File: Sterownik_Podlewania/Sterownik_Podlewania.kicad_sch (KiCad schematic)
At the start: 26 parts, among them J10 Conn_01x06_Socket, J11 Conn_01x06_Socket, J3 Conn_01x05_Pin, J4 Conn_01x05_Pin, J5 Conn_01x03_Pin, J7 Conn_01x05_Socket, J8 Conn_01x04_Socket, J9 Conn_01x06_Socket, U1 ESP32-DEVKITC

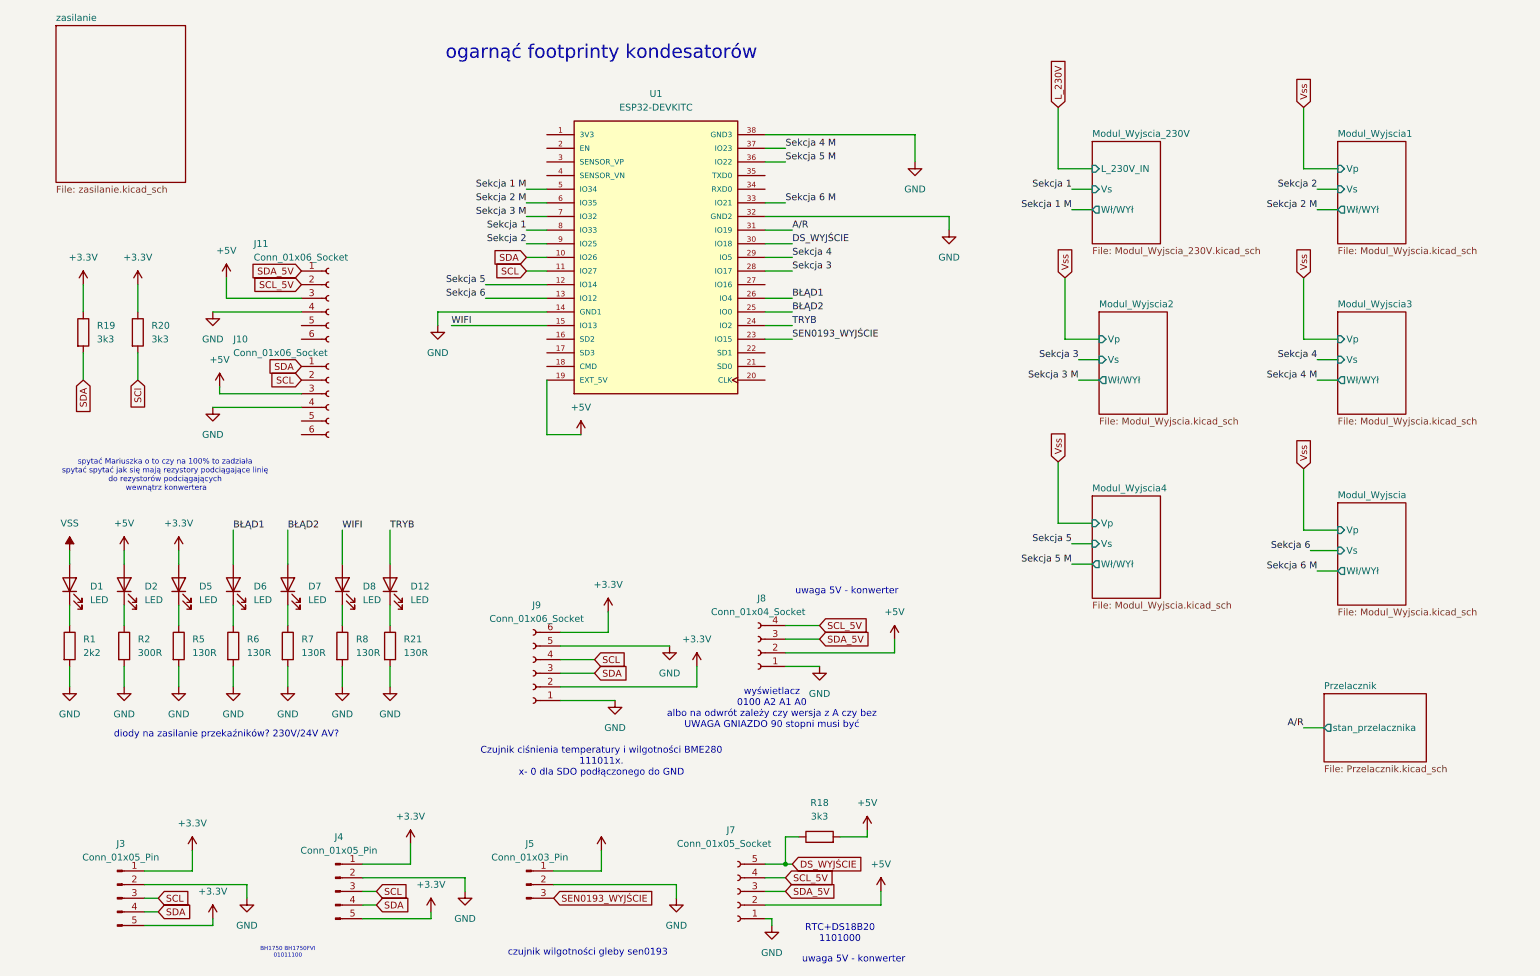
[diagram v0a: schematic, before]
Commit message: Poprawki estetyczne schematu
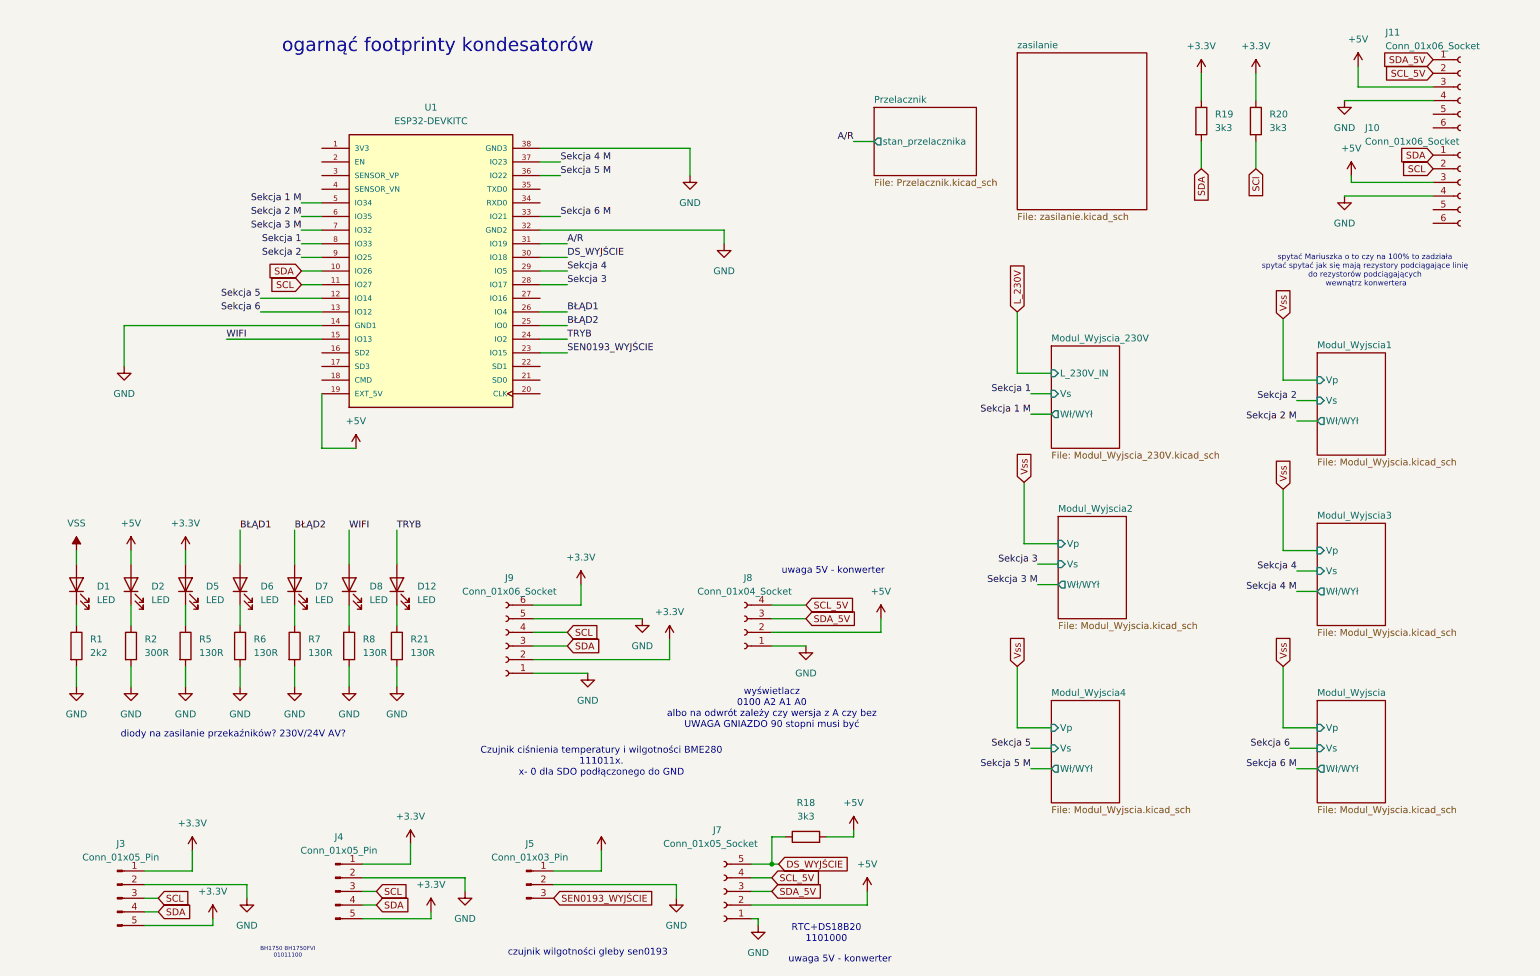
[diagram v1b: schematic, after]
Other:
- title: (none) -> Sterownik podlewania
- moved on the sheet: D1, D12, D2, D5, D6, D7, D8, J10, J11, J7, J8, J9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
